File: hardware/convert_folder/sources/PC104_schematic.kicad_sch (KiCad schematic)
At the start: 22 parts, among them CN20 PC104_inverted, CN21 PC104, CN22 PC104, CN23 PC104, CN24 PC104, CN25 PC104

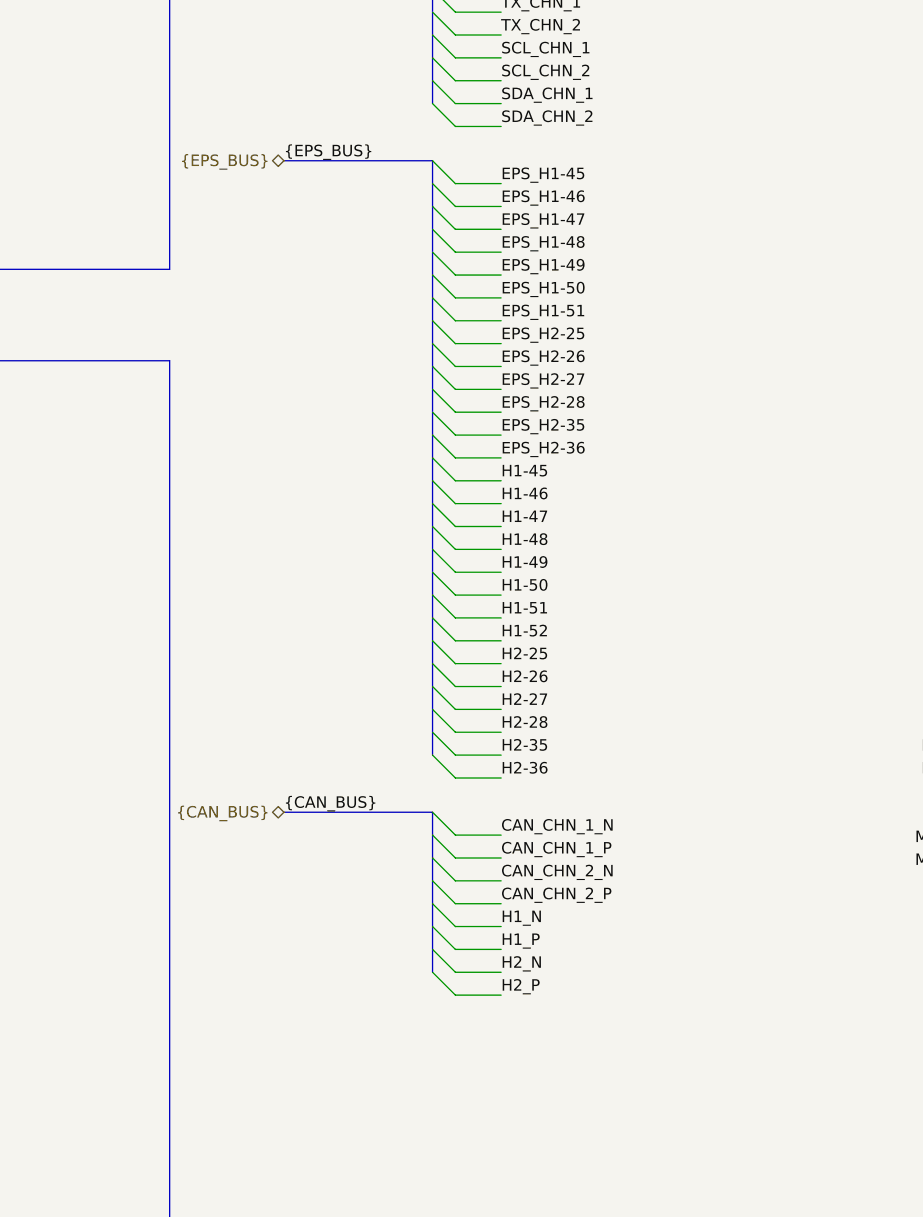
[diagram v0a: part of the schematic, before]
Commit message: fix: start the layout of power path
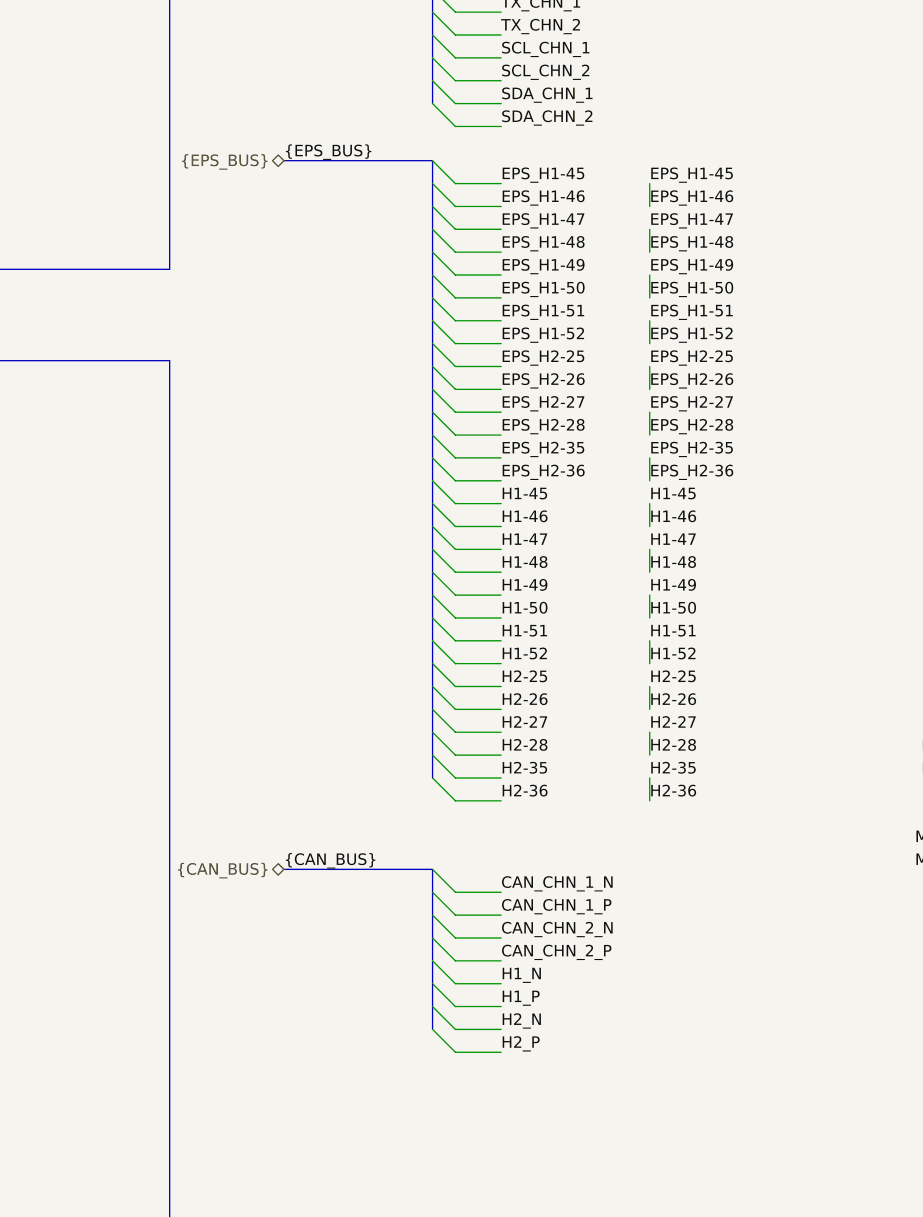
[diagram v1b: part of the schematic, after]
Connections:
- net EPS_H1-46 is gone; now on net EPS_H1-45: CN20.46 (H1-46)
- net EPS_H1-48 is gone; now on net EPS_H1-47: CN20.48 (H1-48)
- net EPS_H1-50 is gone; now on net EPS_H1-49: CN20.50 (H1-50)
- net EPS_H1-52 is gone; now on net EPS_H1-51: CN20.52 (H1-52)
- net EPS_H2-26 is gone; now on net EPS_H2-25: CN20.78 (H2-26)
- net EPS_H2-28 is gone; now on net EPS_H2-27: CN20.80 (H2-28)
- net EPS_H2-36 is gone; now on net EPS_H2-35: CN20.88 (H2-36)
- net H1-46 is gone; now on net H1-45: CN21.46 (H1-46), CN22.46 (H1-46), CN23.46 (H1-46), CN24.46 (H1-46), CN25.46 (H1-46)
- net H1-48 is gone; now on net H1-47: CN21.48 (H1-48), CN22.48 (H1-48), CN23.48 (H1-48), CN24.48 (H1-48), CN25.48 (H1-48)
- net H1-50 is gone; now on net H1-49: CN21.50 (H1-50), CN22.50 (H1-50), CN23.50 (H1-50), CN24.50 (H1-50), CN25.50 (H1-50)
- net H1-52 is gone; now on net H1-51: CN21.52 (H1-52), CN22.52 (H1-52), CN23.52 (H1-52), CN24.52 (H1-52), CN25.52 (H1-52)
- net H2-26 is gone; now on net H2-25: CN21.78 (H2-26), CN22.78 (H2-26), CN23.78 (H2-26), CN24.78 (H2-26), CN25.78 (H2-26)
- net H2-28 is gone; now on net H2-27: CN21.80 (H2-28), CN22.80 (H2-28), CN23.80 (H2-28), CN24.80 (H2-28), CN25.80 (H2-28)
- net H2-36 is gone; now on net H2-35: CN21.88 (H2-36), CN22.88 (H2-36), CN23.88 (H2-36), CN24.88 (H2-36), CN25.88 (H2-36)
